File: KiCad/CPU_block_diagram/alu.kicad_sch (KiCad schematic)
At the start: 30 parts, among them U16 74LS245, U17 74LS283, U18 74LS283, U19 74LS86, U20 74LS86, U21 74LS02, U22 74LS08, U23 74LS173

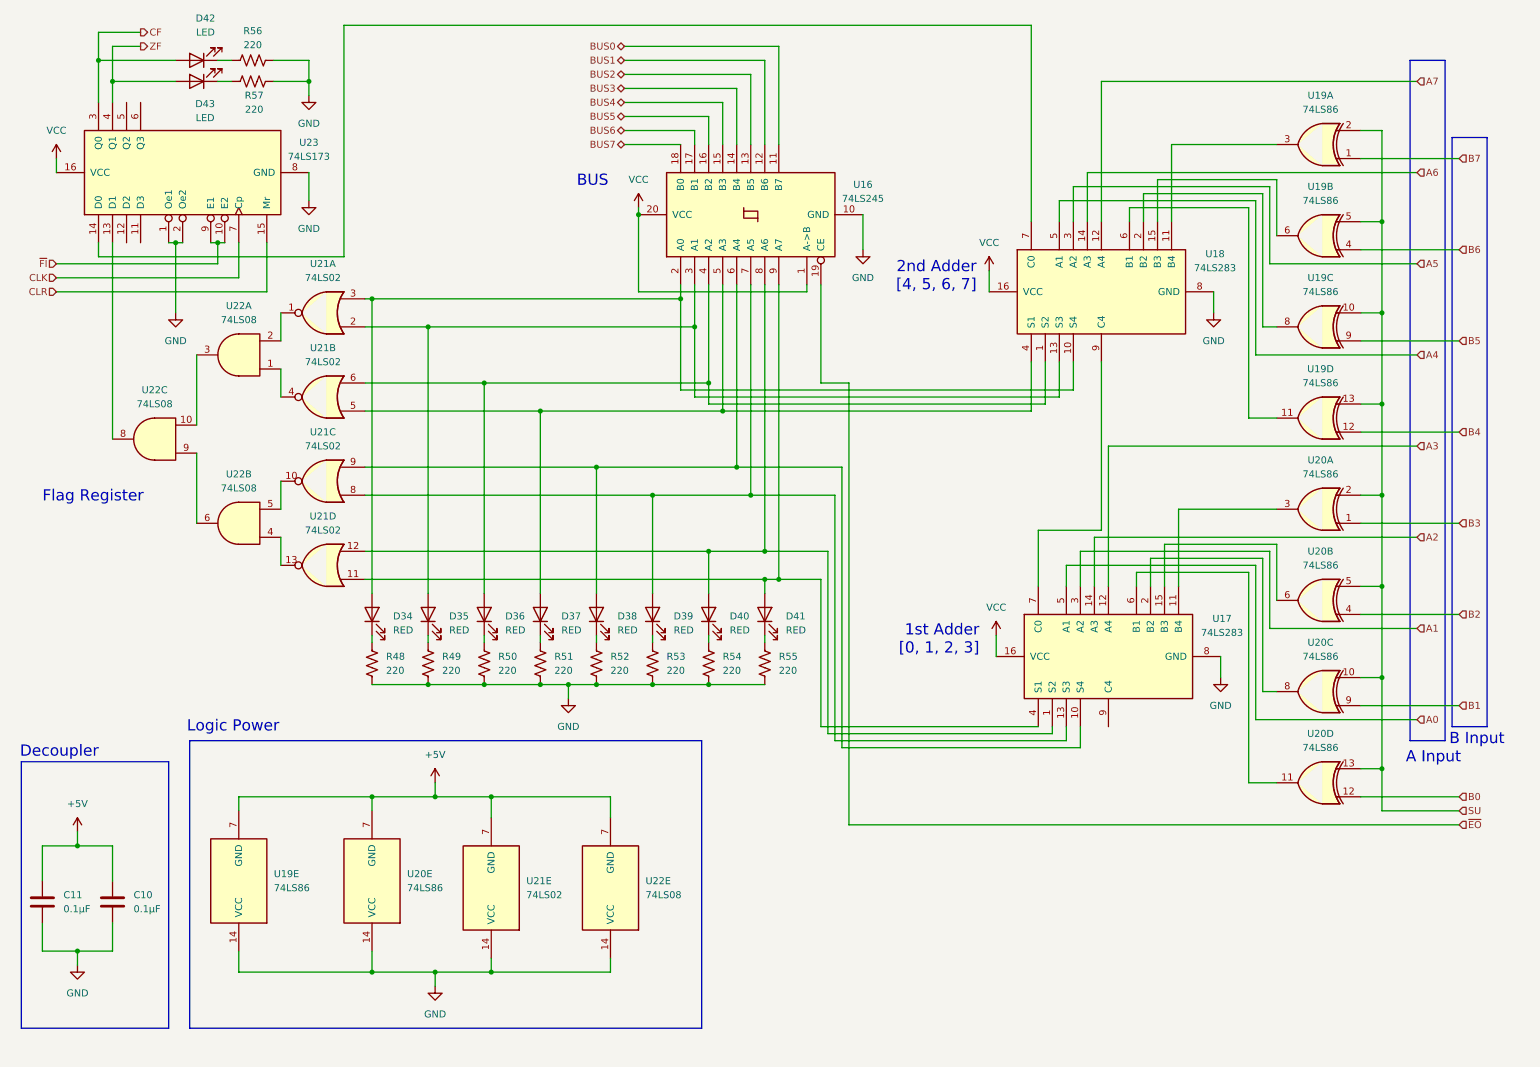
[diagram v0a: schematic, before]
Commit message: vault backup: 2026-01-25 03:55:07
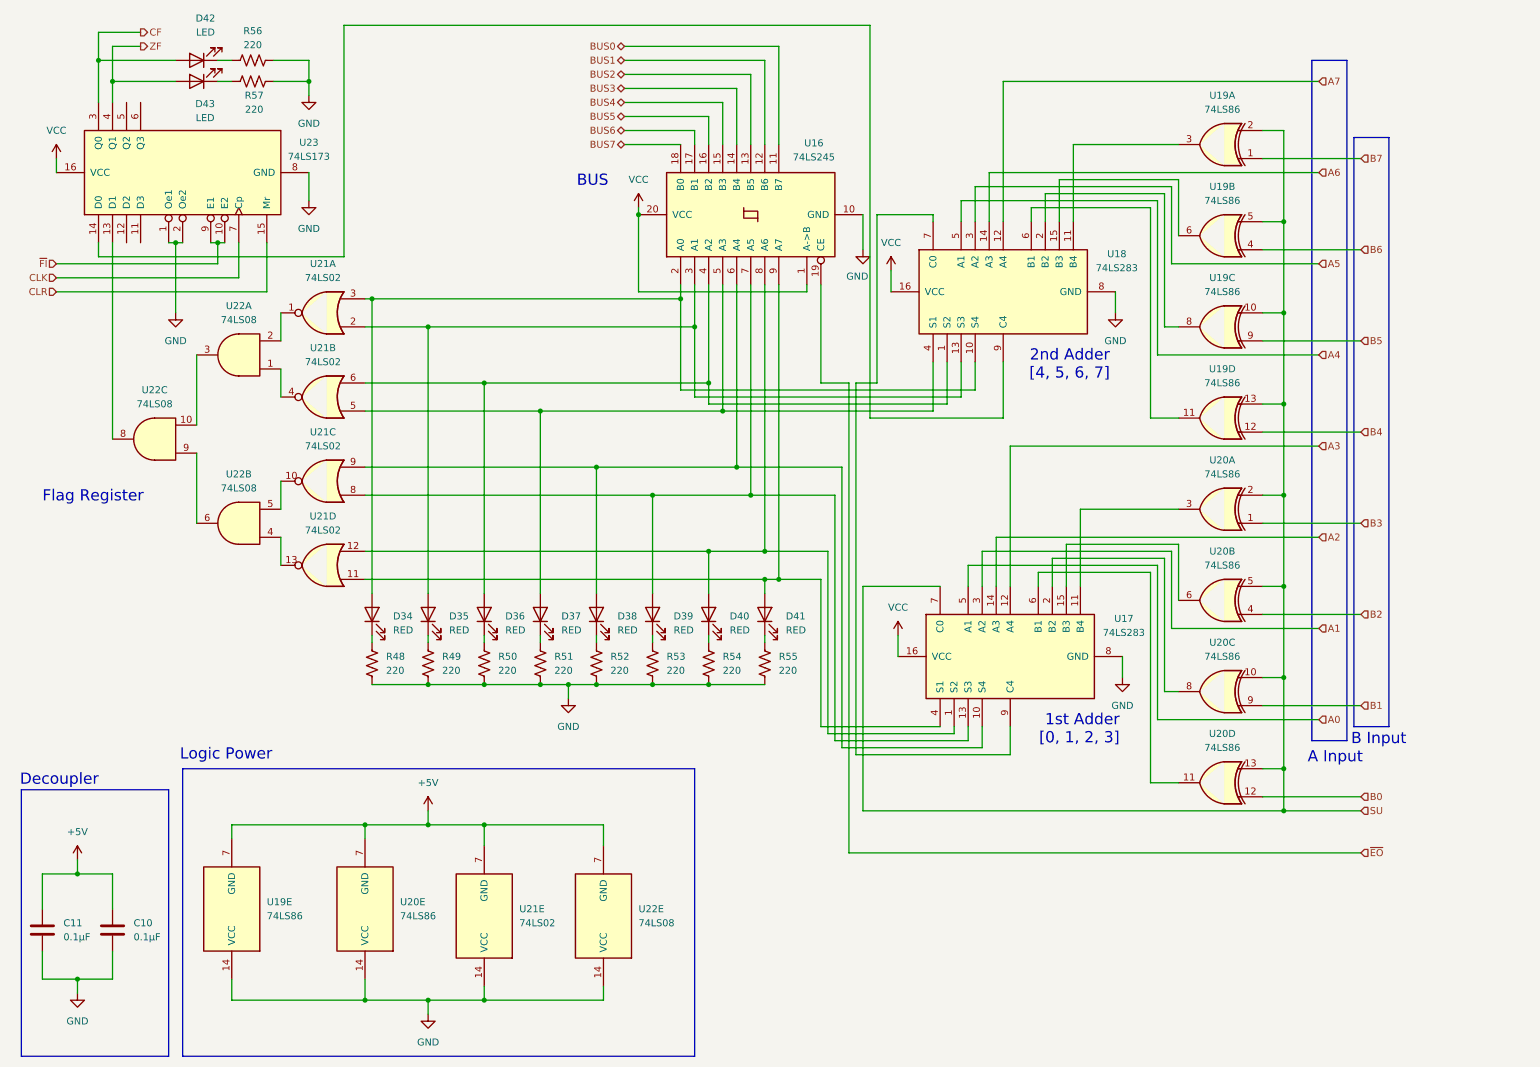
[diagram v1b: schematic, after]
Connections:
- net SU: now also U17.7 (C0)
- net at U18.7 (C0): now also U17.9 (C4); no longer U23.14 (D0)
- net at U18.9 (C4): now also U23.14 (D0); no longer U17.7 (C0)
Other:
- moved on the sheet: C10, C11, U17, U18, U19A, U19B, U19C, U19D, U19E, U20A, U20B, U20C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
